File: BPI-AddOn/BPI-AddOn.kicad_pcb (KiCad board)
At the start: 2 copper layers, 100 x 100 mm, 84 parts, among them CON1 BARREL_JACK, J1 RJ45, J2 RJ45, J3 RJ45, P1 DIN10-1, P10 CONN_01X03, P11 CONN_01X05, P12 CONN_01X05, P13 CONN_01X08, P15 CONN_02X11, P16 USB_B, P17 CONN_01X05, P18 CONN_01X05, P19 V, P2 DIN10-2, P20 - +, P21 USB_OTG, P22 CONN_01X06, P23 CONN_01X06, P24 CONN_02X02, P25 CONN_01X02, P3 DIN10-3, P4 DIN10-4, P5 DIN10-5, P6 DIN7-1, P7 DIN7-2, P8 DIN7-3, P9 CONN_01X03, U1 MC34063, U2 FT230XS

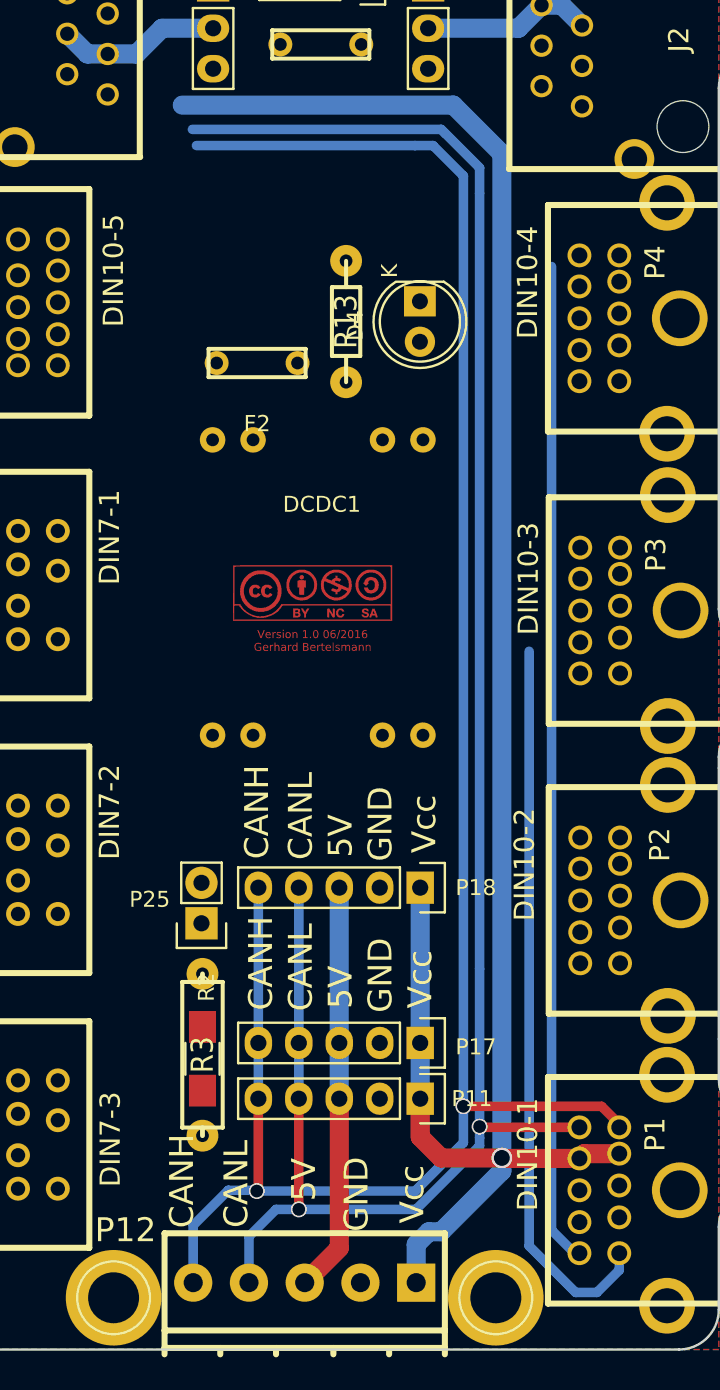
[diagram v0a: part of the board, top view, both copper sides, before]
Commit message: wip
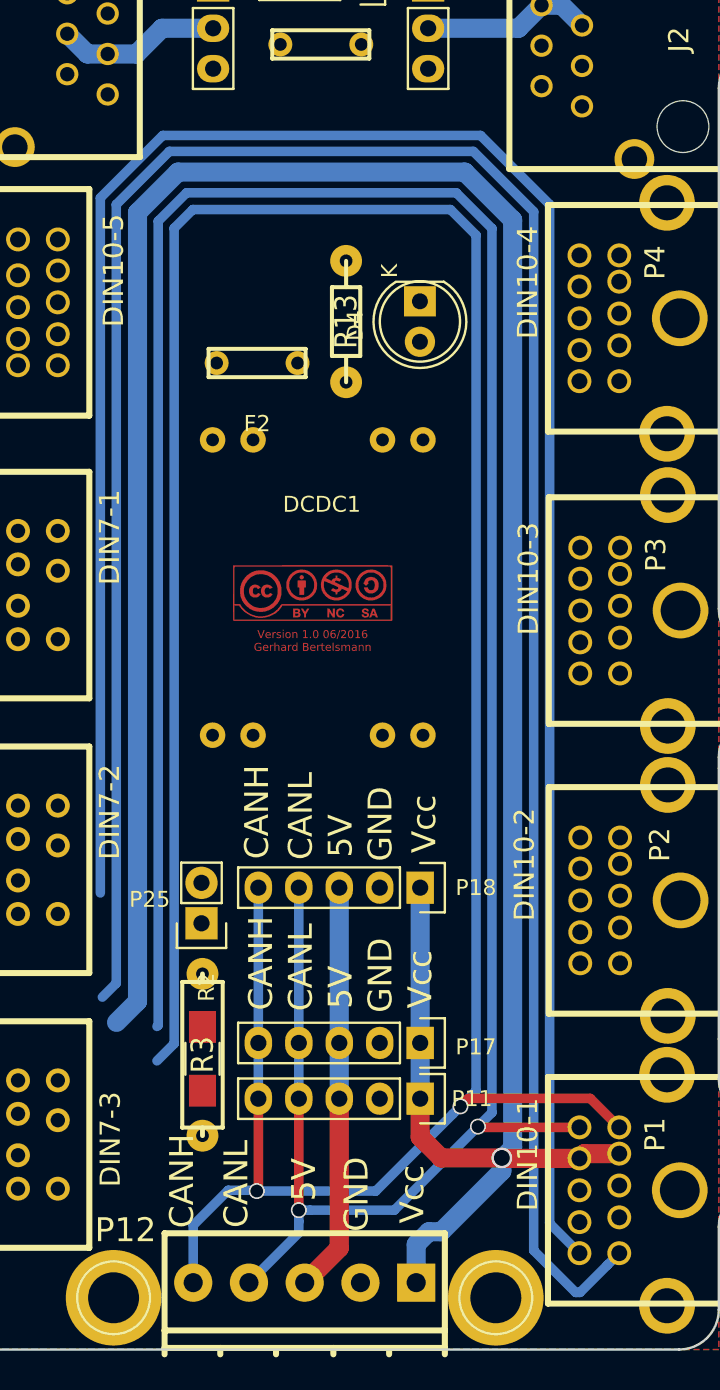
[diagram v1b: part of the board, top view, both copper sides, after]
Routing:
- net /GS0: track 45.8 -> 152.0 mm
- net /GSB: track 62.9 -> 141.9 mm
- net VCC: track 124.4 -> 176.6 mm
- net /CANH: track 130.7 -> 181.6 mm
- net /CANL: track 126.7 -> 175.9 mm
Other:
- net class Defaul_II: clearance 0.2 -> 0.4
- net class Default: clearance 0.2 -> 0.4
- rule trace_clearance: 0.2 -> 0.4
